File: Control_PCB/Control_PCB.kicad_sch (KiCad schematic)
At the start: 0 parts

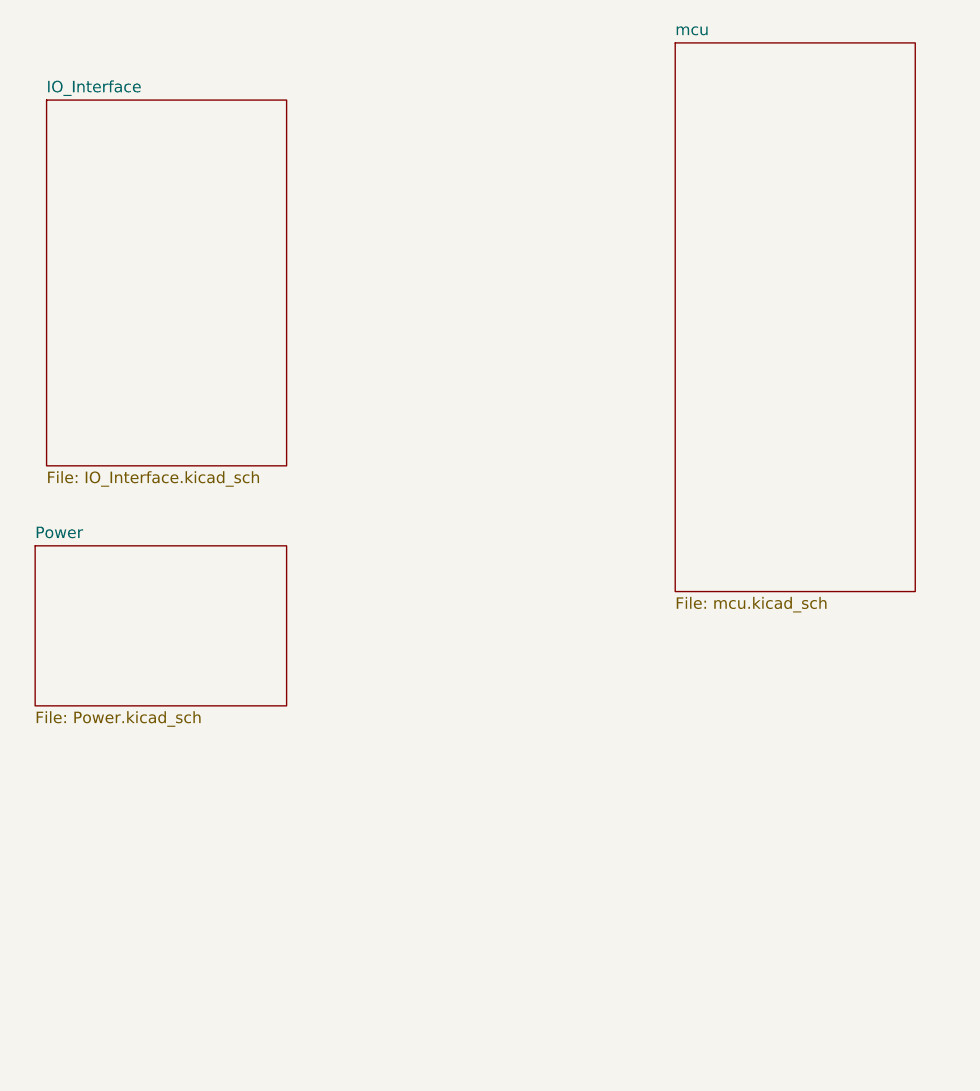
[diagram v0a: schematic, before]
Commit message: 07-20-2026
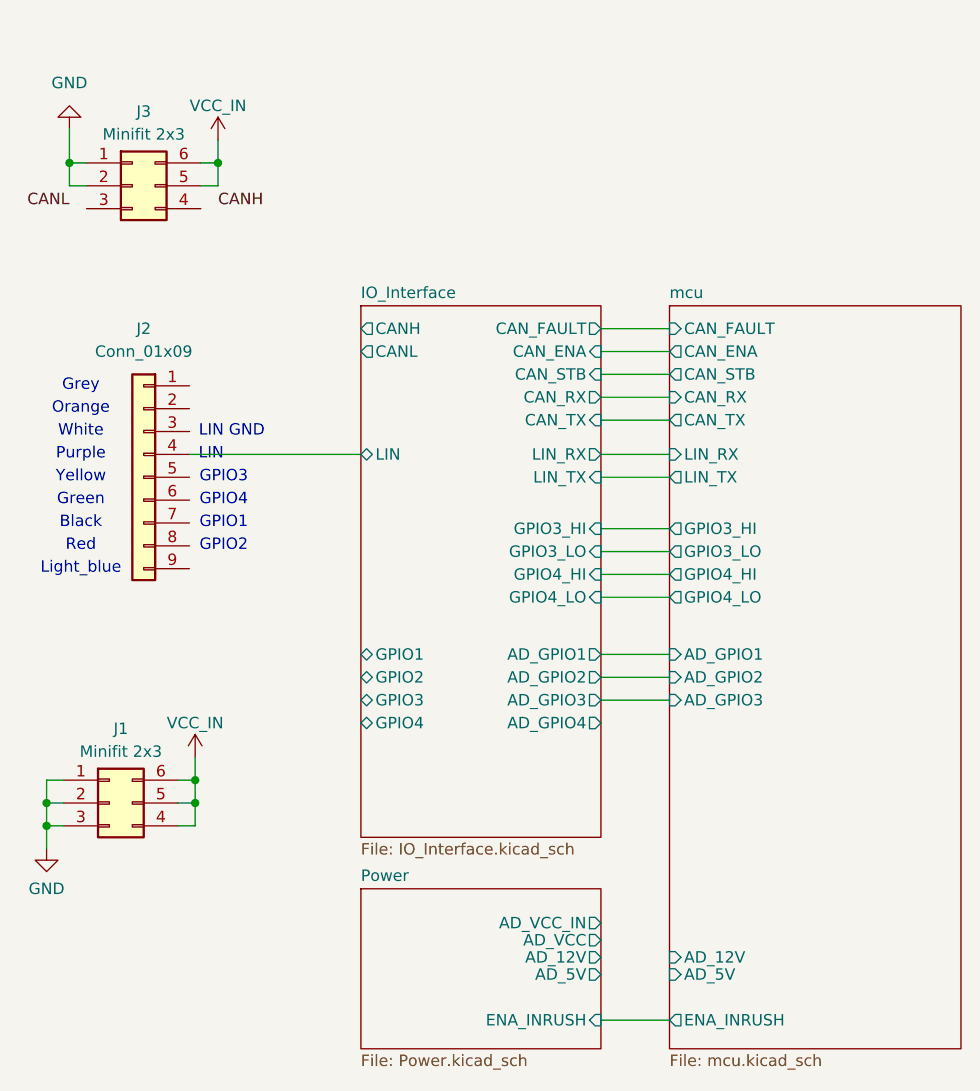
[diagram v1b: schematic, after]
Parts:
- added J1, J3: Minifit 2x3, Connector_Molex:Molex_Mini-Fit_Jr_5569-06A2_2x03_P4.20mm_Horizontal, symbol Connector_Generic:Conn_02x03_Counter_Clockwise
- added J2: Conn_01x09, symbol Connector_Generic:Conn_01x09
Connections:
- new net GND: J1.1 (Pin_1), J1.2 (Pin_2), J1.3 (Pin_3), J3.1 (Pin_1), J3.2 (Pin_2)
- new net IO_Interface/LIN: J2.4 (Pin_4)
- new net VCC_IN: J1.4 (Pin_4), J1.5 (Pin_5), J1.6 (Pin_6), J3.5 (Pin_5), J3.6 (Pin_6)
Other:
- sheet IO_Interface ports: added AD_GPIO1, AD_GPIO2, AD_GPIO3, AD_GPIO4, CANH, CANL, CAN_ENA, CAN_FAULT, CAN_RX, CAN_STB, CAN_TX, GPIO1, GPIO2, GPIO3, GPIO3_HI, GPIO3_LO, GPIO4, GPIO4_HI, GPIO4_LO, LIN, LIN_RX, LIN_TX; removed none
- sheet Power ports: added AD_12V, AD_5V, AD_VCC, AD_VCC_IN, ENA_INRUSH; removed none
- sheet mcu ports: added AD_12V, AD_5V, AD_GPIO1, AD_GPIO2, AD_GPIO3, CAN_ENA, CAN_FAULT, CAN_RX, CAN_STB, CAN_TX, ENA_INRUSH, GPIO3_HI, GPIO3_LO, GPIO4_HI, GPIO4_LO, LIN_RX, LIN_TX; removed none
- note added: "Black"
- note added: "GPIO1"
- note added: "GPIO2"
- note added: "GPIO3"
- note added: "GPIO4"
- note added: "Green"
- note added: "Grey"
- note added: "LIN"
- note added: "LIN GND"
- note added: "Light_blue"
- note added: "Orange"
- note added: "Purple"
- note added: "Red"
- note added: "White"
- note added: "Yellow"
